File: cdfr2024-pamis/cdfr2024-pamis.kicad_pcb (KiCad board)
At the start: 4 copper layers, 75.7 x 64.3 mm, 13 parts, among them J1 Connecteur batterie, J5 Connecteur ToF, J6 Moteur Droit, J7 Moteur Gauche, U2 LM317_SOT-223, U3 ESP32-S3-DEVKITC-1-N8R2, U4 Driver Moteur Droit, U5 Driver Moteur Gauche

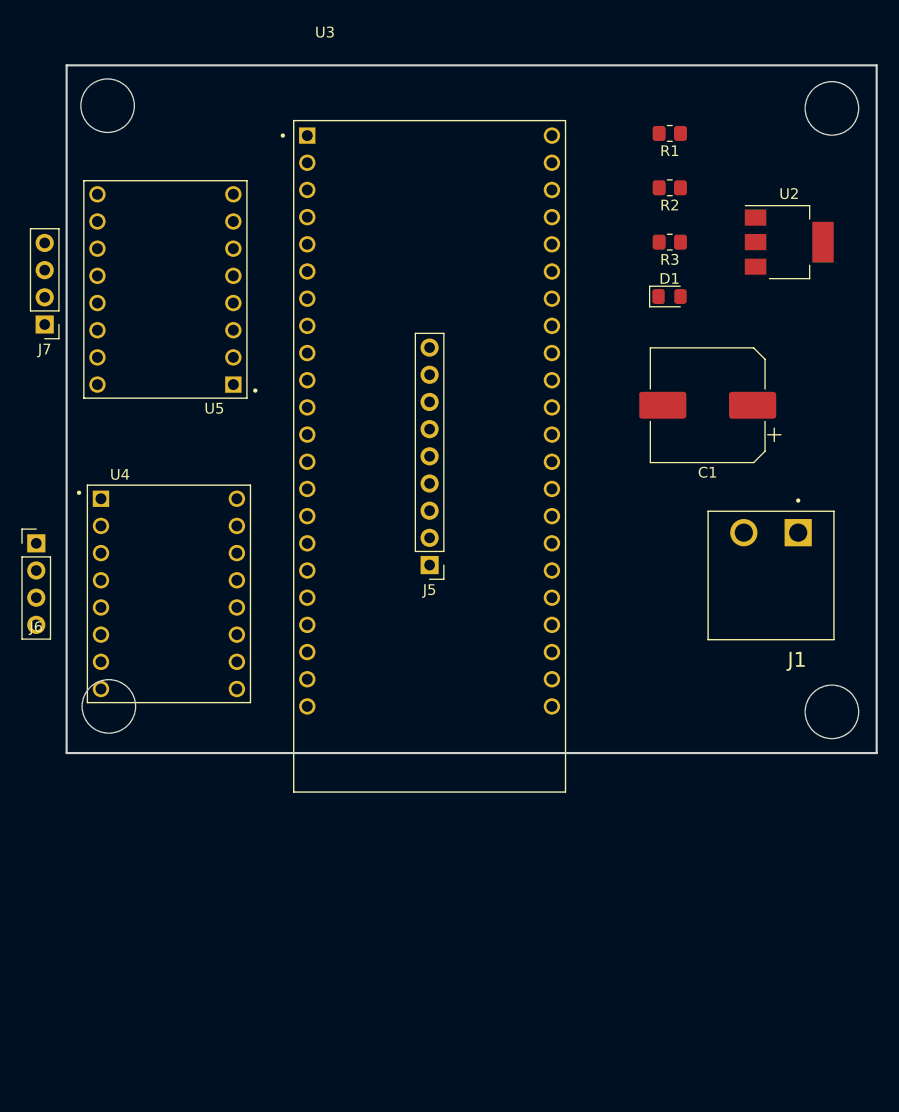
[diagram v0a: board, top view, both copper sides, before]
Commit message: Routage + DRC
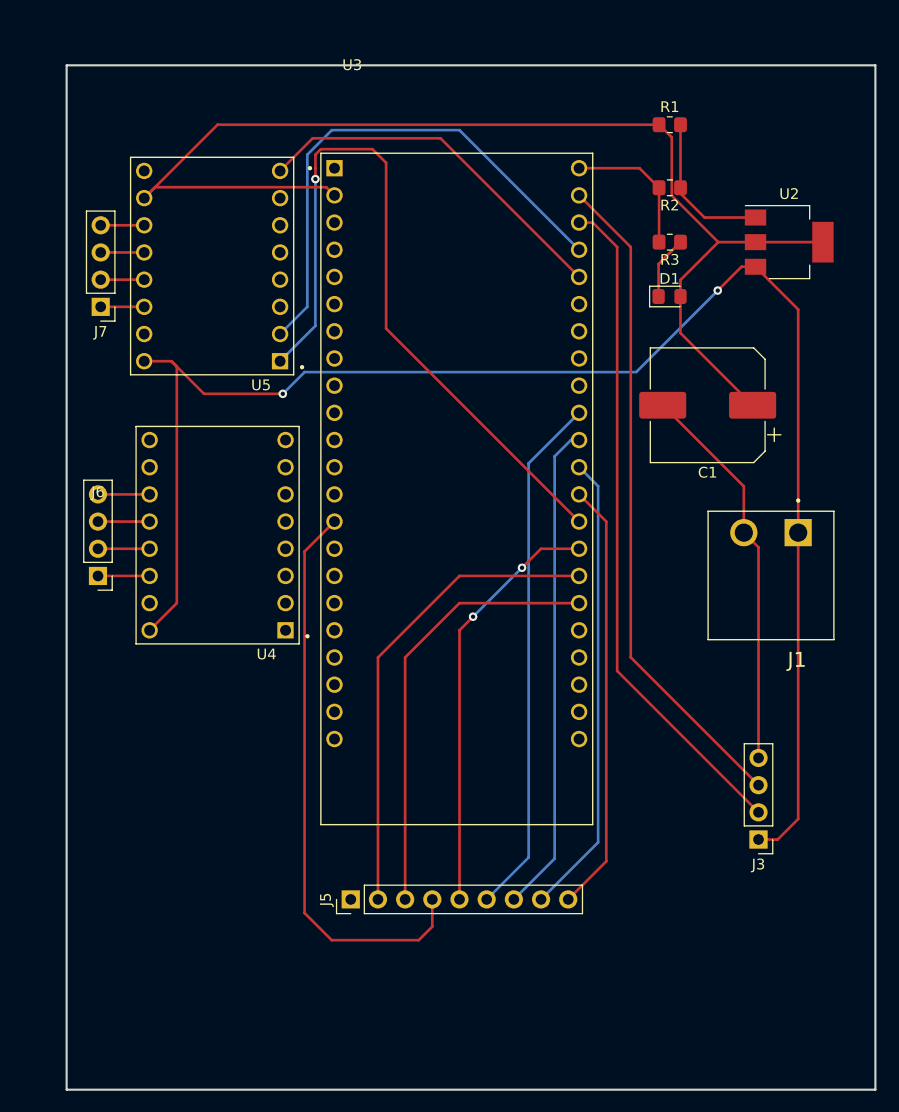
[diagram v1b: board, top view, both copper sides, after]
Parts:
- added J3: Connecteur RF, Connector_PinHeader_2.54mm:PinHeader_1x04_P2.54mm_Vertical, F.Cu at (115.8, 103.9)
- moved J5 32.1 mm to (77.7, 109.5), turned to 90 degrees
- moved U4 7.13 mm to (65.3, 75.4), turned to 180 degrees
- moved J6 6.52 mm to (54.1, 79.2), turned to 180 degrees
- moved J7 5.49 mm to (54.4, 54.1)
- moved U5 4.88 mm to (64.8, 50.3)
- moved U3 3.97 mm to (87.6, 71.1)
- moved R1 0.81 mm to (107.5, 37.1), turned to 0 degrees
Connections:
- U3 pad J1_13: Net-(U3-GPIO3) -> unconnected-(U3-GPIO3-PadJ1_13)
- U3 pad J1_15: Net-(U3-GPIO9) -> unconnected-(U3-GPIO9-PadJ1_15)
- U3 pad J1_16: Net-(U3-GPIO10) -> unconnected-(U3-GPIO10-PadJ1_16)
- U3 pad J1_20: Net-(U3-GPIO14) -> unconnected-(U3-GPIO14-PadJ1_20)
- U3 pad J1_4: Net-(U3-GPIO4) -> unconnected-(U3-GPIO4-PadJ1_4)
- U3 pad J1_5: Net-(U3-GPIO5) -> unconnected-(U3-GPIO5-PadJ1_5)
- U3 pad J3_2: unconnected-(U3-U0TXD/GPIO43-PadJ3_2) -> Net-(J3-Pin_3)
- U3 pad J3_3: unconnected-(U3-U0RXD/GPIO44-PadJ3_3) -> Net-(J3-Pin_2)
- U4 pad 5: Net-(U3-GPIO11) -> unconnected-(U4-M2-Pad5)
- U4 pad 6: Net-(U3-GPIO12) -> unconnected-(U4-M1-Pad6)
- U4 pad 7: Net-(U3-GPIO13) -> unconnected-(U4-M0-Pad7)
- U5 pad 5: Net-(U3-GPIO2) -> unconnected-(U5-M2-Pad5)
- U5 pad 6: Net-(U3-GPIO3) -> unconnected-(U5-M1-Pad6)
- U5 pad 7: Net-(U3-GPIO4) -> unconnected-(U5-M0-Pad7)
- U5 pad 8: Net-(U3-GPIO5) -> Net-(U3-GPIO2)
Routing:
- net +7.5V: track 0.00 -> 147.7 mm, vias 0 -> 2
- net +3.3V: track 0.00 -> 112.0 mm
- net Net-(U3-GPIO0): track 0.00 -> 69.0 mm, vias 0 -> 1
- net Net-(J3-Pin_2): track 0.00 -> 62.8 mm
- net Net-(J3-Pin_3): track 0.00 -> 62.1 mm
- net Net-(J5-Pin_4): track 0.00 -> 53.8 mm
- net GND: track 0.00 -> 50.0 mm
- net Net-(J5-Pin_6): track 0.00 -> 49.0 mm
- net Net-(U3-GPIO1): track 0.00 -> 48.8 mm
- net Net-(J5-Pin_7): track 0.00 -> 45.9 mm
- net Net-(J5-Pin_2): track 0.00 -> 44.6 mm
- net Net-(J5-Pin_8): track 0.00 -> 43.3 mm
- net Net-(J5-Pin_3): track 0.00 -> 41.0 mm
- net Net-(J5-Pin_9): track 0.00 -> 40.4 mm
- net Net-(J5-Pin_5): track 0.00 -> 39.5 mm, vias 0 -> 2
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- added copper zone on In2.Cu, net +3.3V
- added copper zone on In1.Cu, net GND
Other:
- board size 75.7 x 64.3 mm -> 75.6 x 95.7 mm
